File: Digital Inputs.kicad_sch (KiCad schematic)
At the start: 3 parts, among them J5 Screw_Terminal_01x06, J6 Screw_Terminal_01x06, J7 Screw_Terminal_01x06

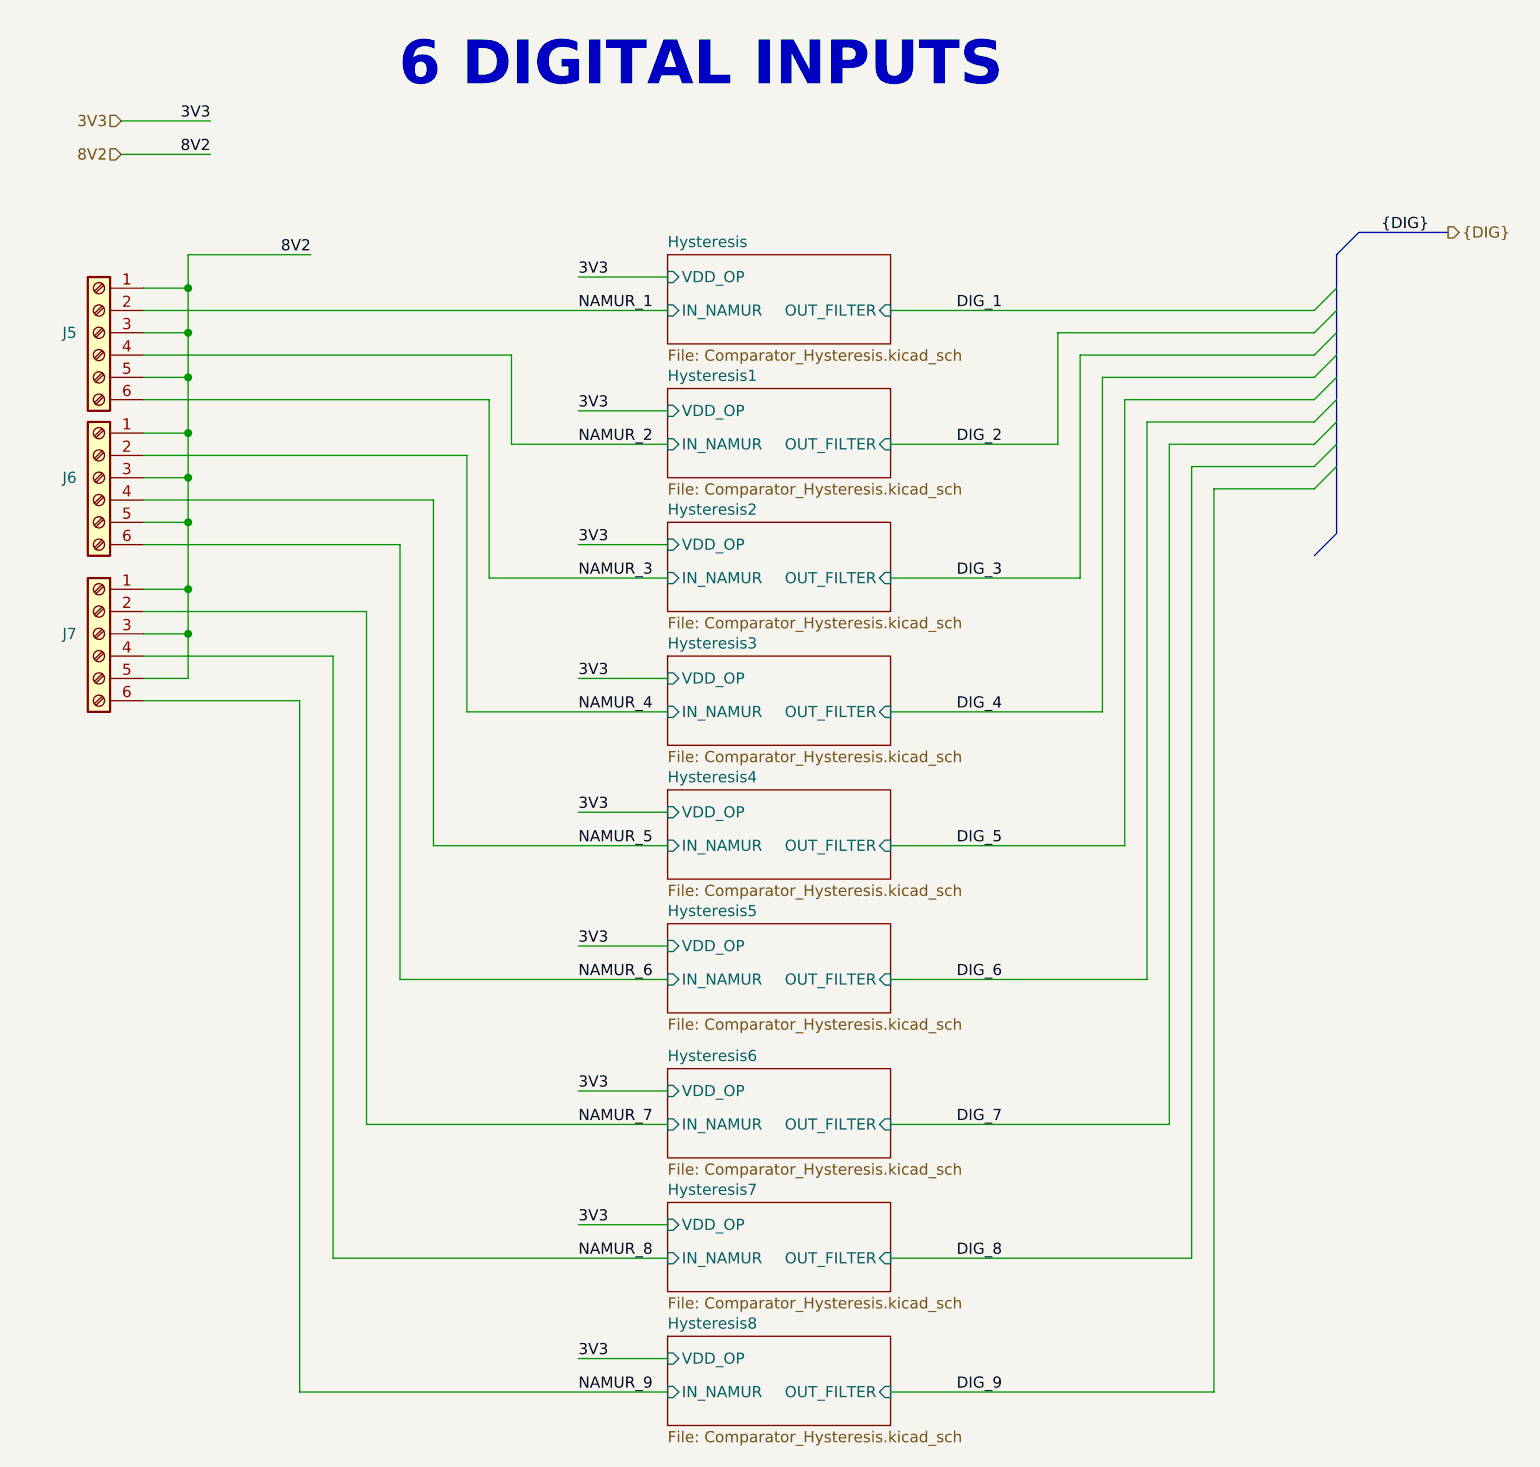
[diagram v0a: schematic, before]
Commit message: Avance del posicionamiento
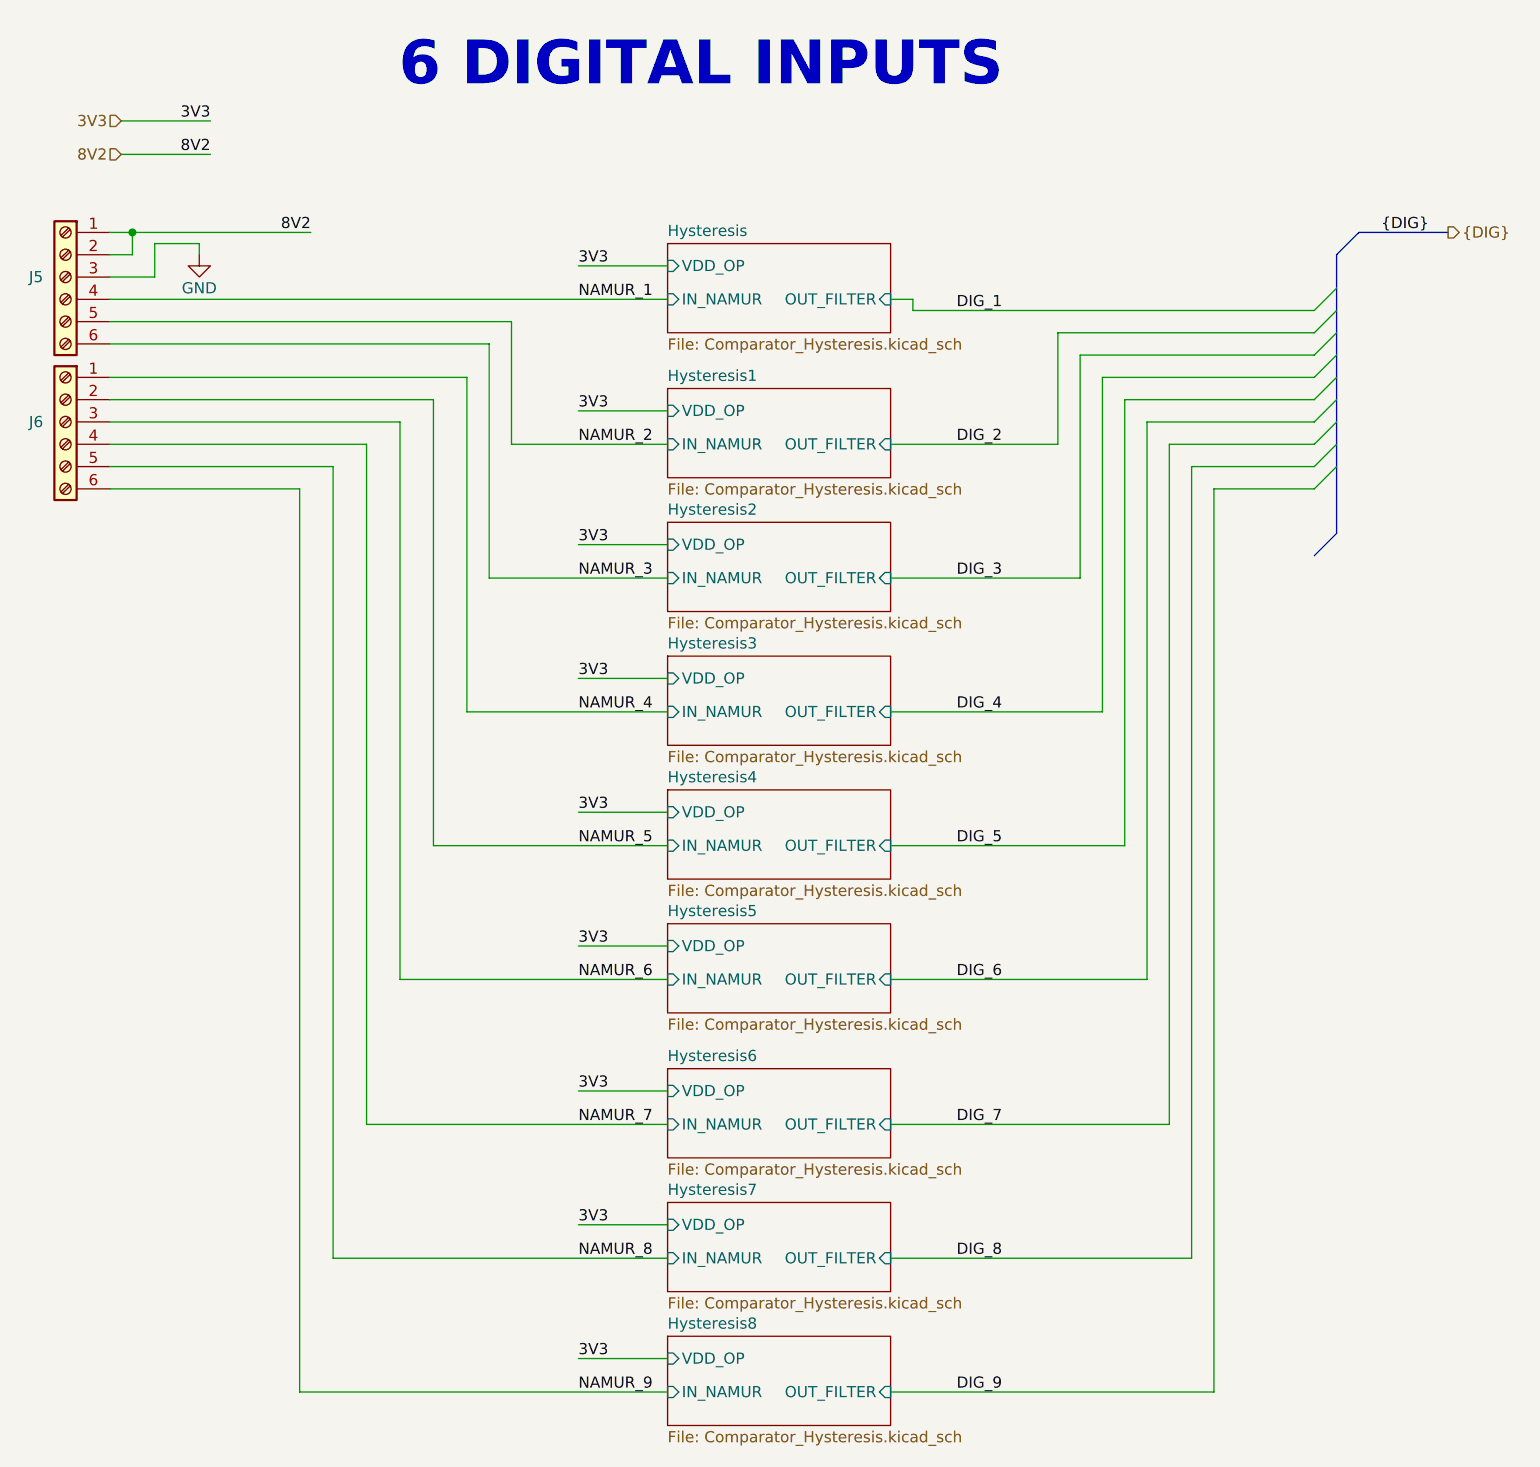
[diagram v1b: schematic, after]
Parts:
- removed J7: Screw_Terminal_01x06, LIB_PCB_CONT:15EDGVC_6P_3.81mm_Male-Vert_Degson, symbol Connector:Screw_Terminal_01x06
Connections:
- net 8V2: now also J5.2 (Pin_2); no longer J5.3 (Pin_3), J5.5 (Pin_5), J6.1 (Pin_1), J6.3 (Pin_3), J6.5 (Pin_5)
- net NAMUR_1: now also J5.4 (Pin_4); no longer J5.2 (Pin_2)
- net NAMUR_2: now also J5.5 (Pin_5); no longer J5.4 (Pin_4)
- net NAMUR_4: now also J6.1 (Pin_1); no longer J6.2 (Pin_2)
- net NAMUR_5: now also J6.2 (Pin_2); no longer J6.4 (Pin_4)
- net NAMUR_6: now also J6.3 (Pin_3); no longer J6.6 (Pin_6)
- net NAMUR_7: now also J6.4 (Pin_4)
- net NAMUR_8: now also J6.5 (Pin_5)
- net NAMUR_9: now also J6.6 (Pin_6)
- new net GND: J5.3 (Pin_3)
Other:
- moved on the sheet: J5, J6
